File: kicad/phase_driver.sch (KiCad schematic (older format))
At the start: 15 parts, among them Q11 IRF3205, Q2 IRF3205, Q5 IRF3205, Q8 IRF3205, U3 MIC4605

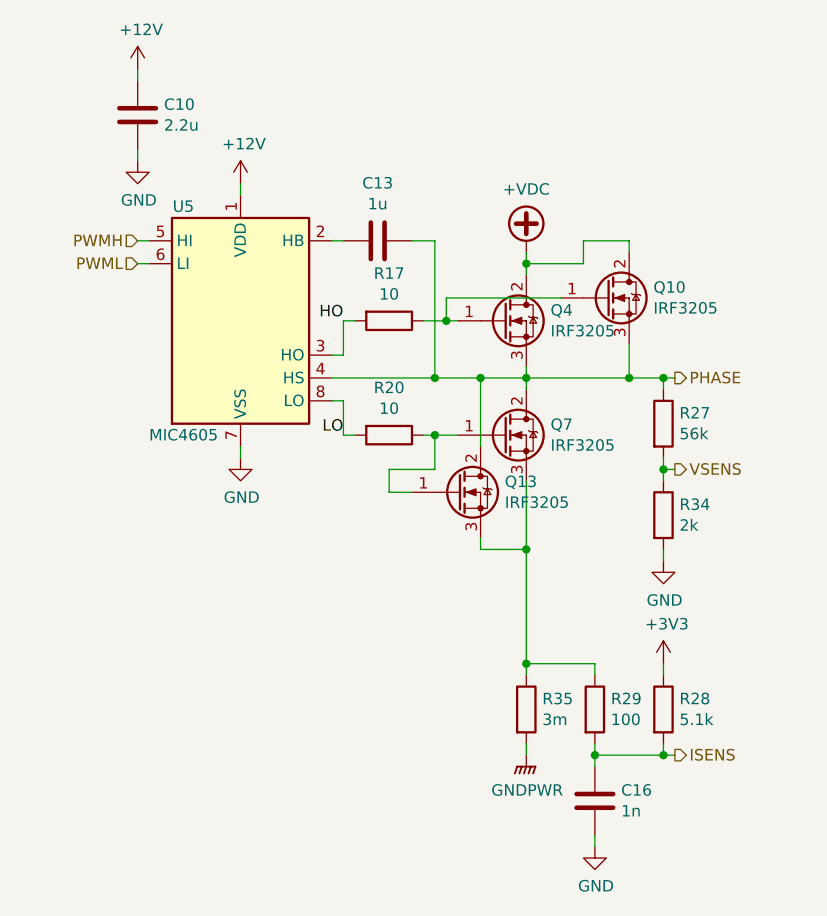
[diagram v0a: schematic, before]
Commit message: added finished adding MPNs to all components
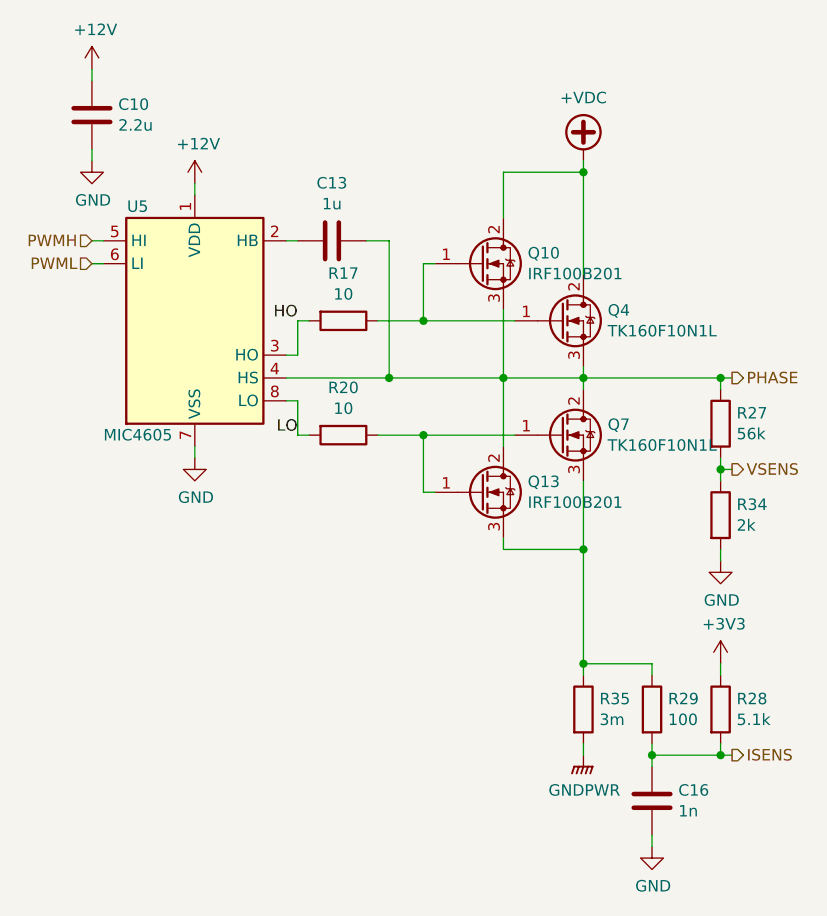
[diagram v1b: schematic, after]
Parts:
- C11: MPN (none) -> 885012106022
- C14: MPN (none) -> 885012206083
- C8: MPN (none) -> GRM188R61E225MA12D; Voltage Rating DC 16 -> 25
- Q11, Q8: value IRF3205 -> IRF100B201; MPN (none) -> IRF100B201
- Q2, Q5: value IRF3205 -> TK160F10N1L; MPN (none) -> TK160F10N1L,LQ
- R15, R18: MPN (none) -> RC0603FR-0710RP
- R21: MPN (none) -> RC0603FR-0756KL
- R22: MPN (none) -> RC0603FR-075K1L
- R23: MPN (none) -> RC0603FR-07100RL
- R30: MPN (none) -> RC0603FR-072KL
- R31: MPN (none) -> WSLF25123L000FEA
- U3: MPN (none) -> MIC4605-1YM-TR
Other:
- moved on the sheet: C10, C13, C16, Q10, Q13, Q4, Q7, R17, R20, R27, R28, R29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
